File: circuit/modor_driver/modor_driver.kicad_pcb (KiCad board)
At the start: 2 copper layers, 50 x 50 mm, 26 parts, among them J1 ZH, J2 ZH, J3 pogo pin, J4 PH, J5 XH, J6 PA, J7 XT_pad, J8 XT_pad, SW1 SW_Push, U2 STM32C011F4Px

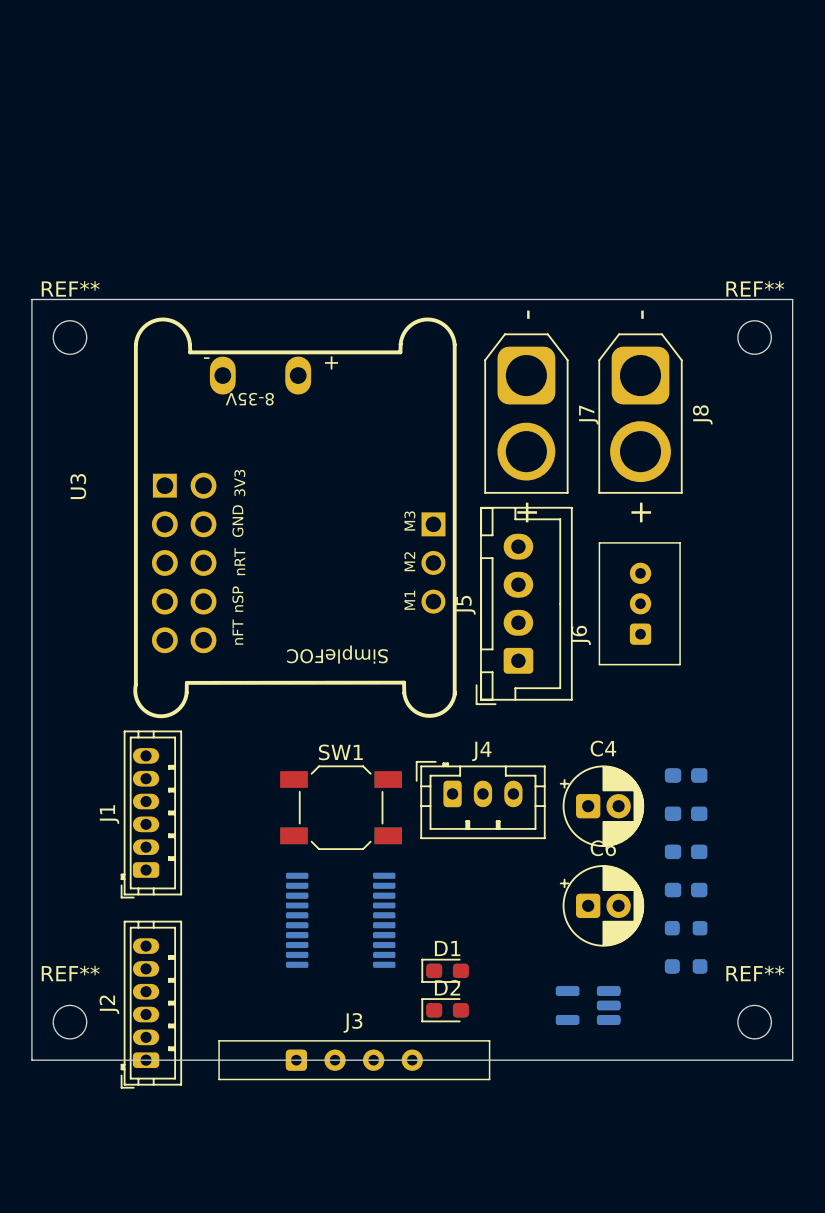
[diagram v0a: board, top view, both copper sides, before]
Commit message: レイアウト
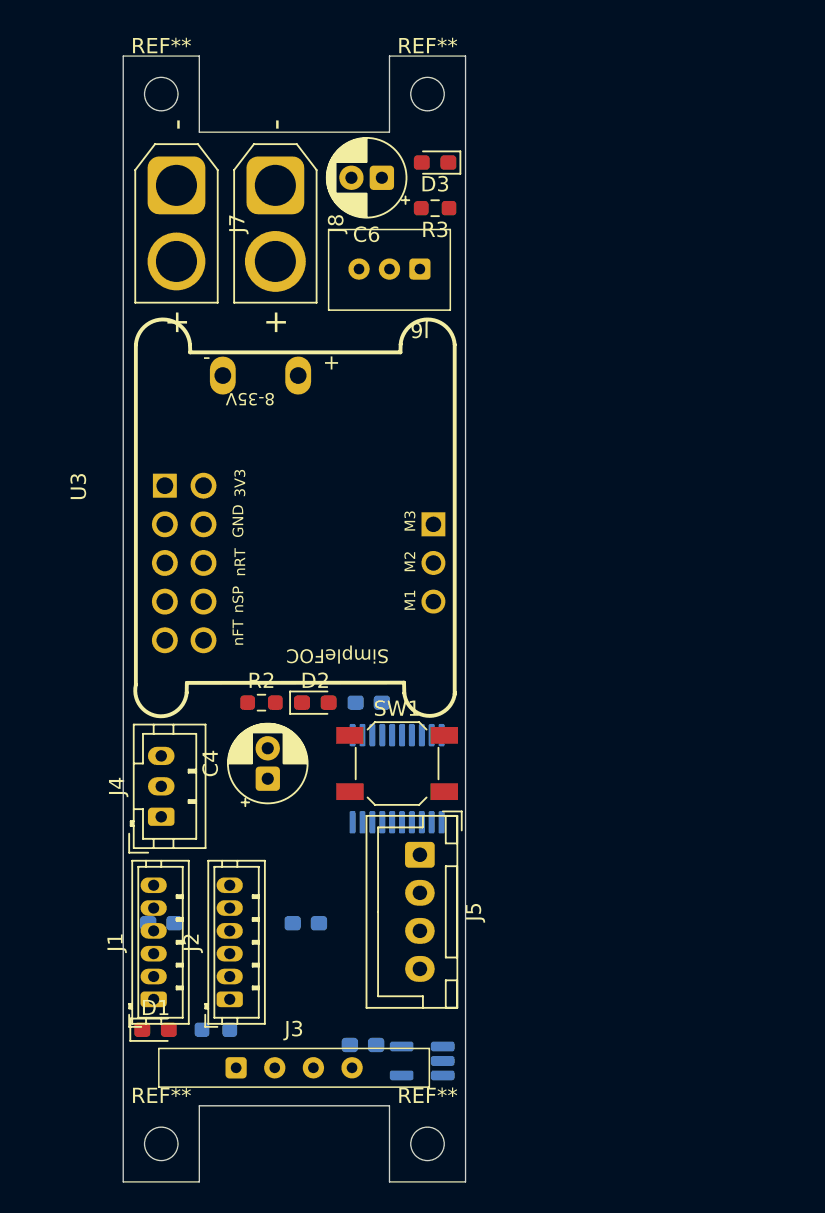
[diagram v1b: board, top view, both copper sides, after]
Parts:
- added D3: LED_Small, LED_SMD:LED_0603_1608Metric_Pad1.05x0.95mm_HandSolder, F.Cu at (141.5, 61.0)
- added R3: 10k, Resistor_SMD:R_0603_1608Metric_Pad0.98x0.95mm_HandSolder, F.Cu at (141.5, 64.0)
- R2: moved to F.Cu
- moved C6 49.7 mm to (138.0, 62.0), turned to 180 degrees
- moved C1 35.8 mm to (123.5, 111.0)
- moved R2 32.9 mm to (130.1, 96.5), turned to 0 degrees
- moved R1 31.6 mm to (127.1, 118.0)
- moved J6 28.0 mm to (140.5, 68.0), turned to 180 degrees
- moved J8 27.1 mm to (131.0, 62.5)
- moved REF** 26.8 mm to (141.0, 56.5)
- moved J7 26.2 mm to (124.5, 62.5)
- moved C2 26.1 mm to (136.8, 119.0)
- moved C3 25.4 mm to (133.0, 111.0)
- moved C5 24.2 mm to (137.1, 96.5)
- moved REF** 22.9 mm to (141.0, 125.5)
- moved D2 22.0 mm to (133.6, 96.5)
- moved C4 21.1 mm to (130.5, 101.5), turned to 90 degrees
- moved D1 19.6 mm to (123.1, 118.0)
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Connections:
- net Net-(J7-Pin_2) renamed +BATT
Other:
- board size 50 x 50 mm -> 22.5 x 74 mm
